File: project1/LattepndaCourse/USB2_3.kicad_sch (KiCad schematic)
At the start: 0 parts

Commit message: Hierachi
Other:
- title: (none) -> practice design
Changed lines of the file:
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@@
 	(generator "eeschema")
 	(generator_version "9.0")
-	(paper "A4")
+	(paper "A2")
+	(title_block
+		(title "practice design")
+		(date "2026-09-30")
+		(rev "1")
+	)
 )

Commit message: USB is done
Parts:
- added C57, C58: 22uF/10V, A_HDJ_Library:C_0603_1608Metric, symbol Device:C_Small
- added C59, C60, C61, C62: 100nF/50V, A_HDJ_Library:C_0603_1608Metric, symbol Device:C_Small
- added D19, D20, D21, D22: ESD9B5.0ST5G, A_HDJ_Library:D_0402_1005Metric, symbol Diode:ESD9B5.0ST5G
- added F1, F2, F3, F4: 6V/1A, A_HDJ_Library:Fuse_0805_2012Metric, symbol Device:Fuse
- added J17: USB_A_Stacked, A_HDJ_Library:USB_A_CUI_UJ2-ADH-TH_Horizontal_Stacked, symbol Connector:USB_A_Stacked
- added J18: USB3_A_Stacked, A_HDJ_Library:USB3_A_Molex_48406-0001_Horizontal_Stacked, symbol Connector:USB3_A_Stacked
- added U13, U14, U15: ULC0524P, A_HDJ_Library:Diodes_UDFN-10_1.0x2.5mm_P0.5mm, symbol Power_Protection:D3V3XA4B10LP
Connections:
- new net: F3.2, J18.1 (VBUS1)
- new net: F4.2, J18.10 (VBUS2)
- new net: F2.2, J17.5 (VBUS2)
- new net: F1.2, J17.1 (VBUS1)
- new net +5V: C57.1, C57.2, C58.1, C58.2, D19.2 (A2), D20.2 (A2), D21.2 (A2), D22.2 (A2), F1.1, F2.1, F3.1, F4.1, J17.4 (GND1), J17.8 (GND2), J17.SH (Shield), J18.13 (GND2), J18.16 (DRAIN2), J18.4 (GND1), J18.7 (DRAIN1), J18.SH (SHIELD), J18.SH (SHIELD), U13.3 (VSS), U13.8 (VSS), U14.3 (VSS), U14.8 (VSS), U15.3 (VSS), U15.8 (VSS)
- new net CON_USB3_SSTX_N: C59.1, J18.8 (SSTX1-), U15.4, U15.7 (NC)
- new net CON_USB3_SSTX_P: C60.1, J18.9 (SSTX1+), U15.5, U15.6 (NC)
- new net CON_USB4_SSTX_N: C61.1, J18.17 (SSTX2-), U15.1, U15.10 (NC)
- new net CON_USB4_SSTX_P: C62.1, J18.18 (SSTX2+), U15.2, U15.9 (NC)
- new net USB3_SSRT_N: J18.5 (SSRX1-), U14.4, U14.7 (NC)
- new net USB3_SSRT_P: J18.6 (SSRX1+), U14.5, U14.6 (NC)
- new net USB3_SSXT_N: C59.2
- new net USB3_SSXT_P: C60.2
- new net USB4_SSRT_N: J18.14 (SSRX2-), U14.1, U14.10 (NC)
- new net USB4_SSRT_P: J18.15 (SSRX2+), U14.2, U14.9 (NC)
- new net USB4_SSXT_N: C61.2
- new net USB4_SSXT_P: C62.2
- new net USB_2_P1+: J18.12 (D2+)
- new net USB_2_P1-: J18.11 (D2-)
- new net USB_2_P2+: J18.3 (D1+)
- new net USB_2_P2-: J18.2 (D1-)
- new net USB_2_P3+: D21.1 (A1), J17.7 (D2+), U13.4, U13.7 (NC)
- new net USB_2_P3-: D22.1 (A1), J17.6 (D2-), U13.5, U13.6 (NC)
- new net USB_2_P5+: D19.1 (A1), J17.3 (D1+), U13.1, U13.10 (NC)
- new net USB_2_P5-: D20.1 (A1), J17.2 (D1-), U13.2, U13.9 (NC)
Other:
- note added: "ESD Protection diods for USB 2.0 data line"
- note added: "USB 2.0"
- note added: "USB 3.0"

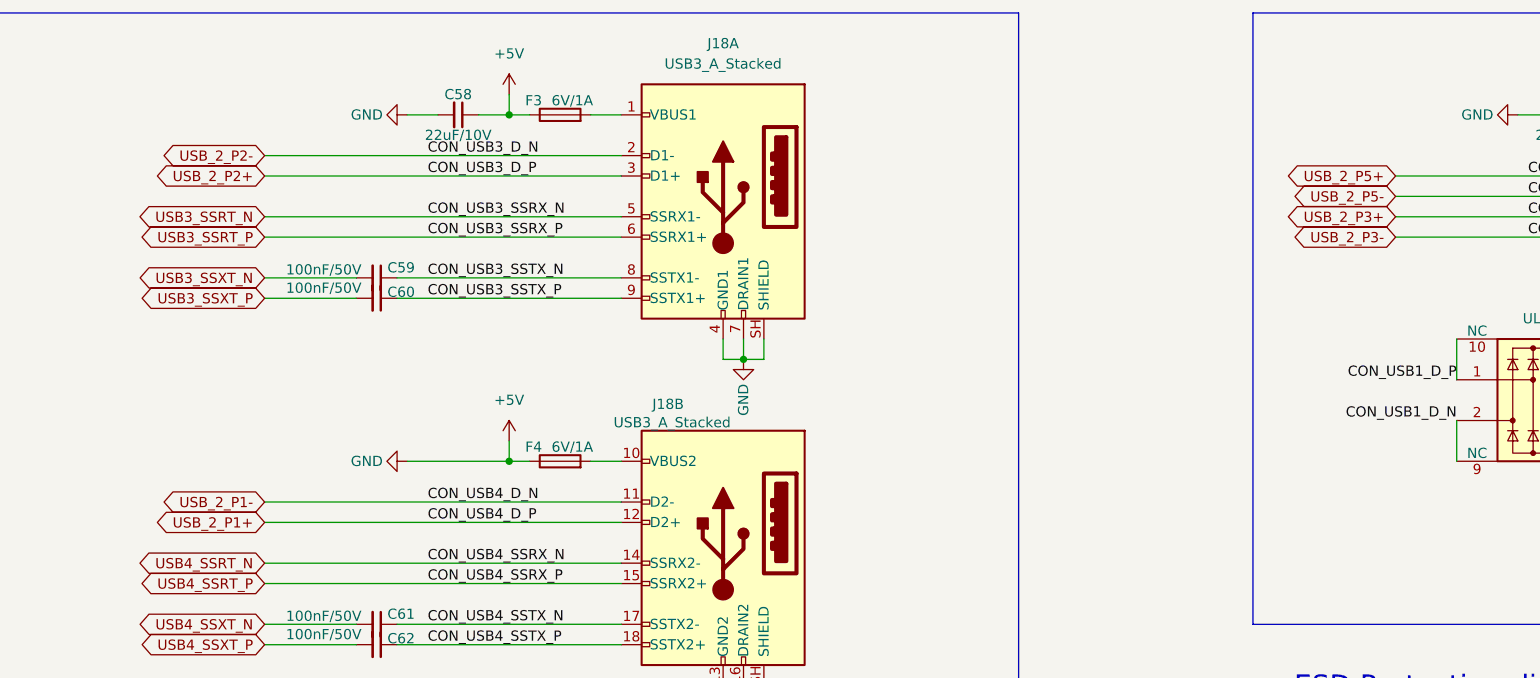
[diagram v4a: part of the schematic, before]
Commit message: Hierachi needs some work
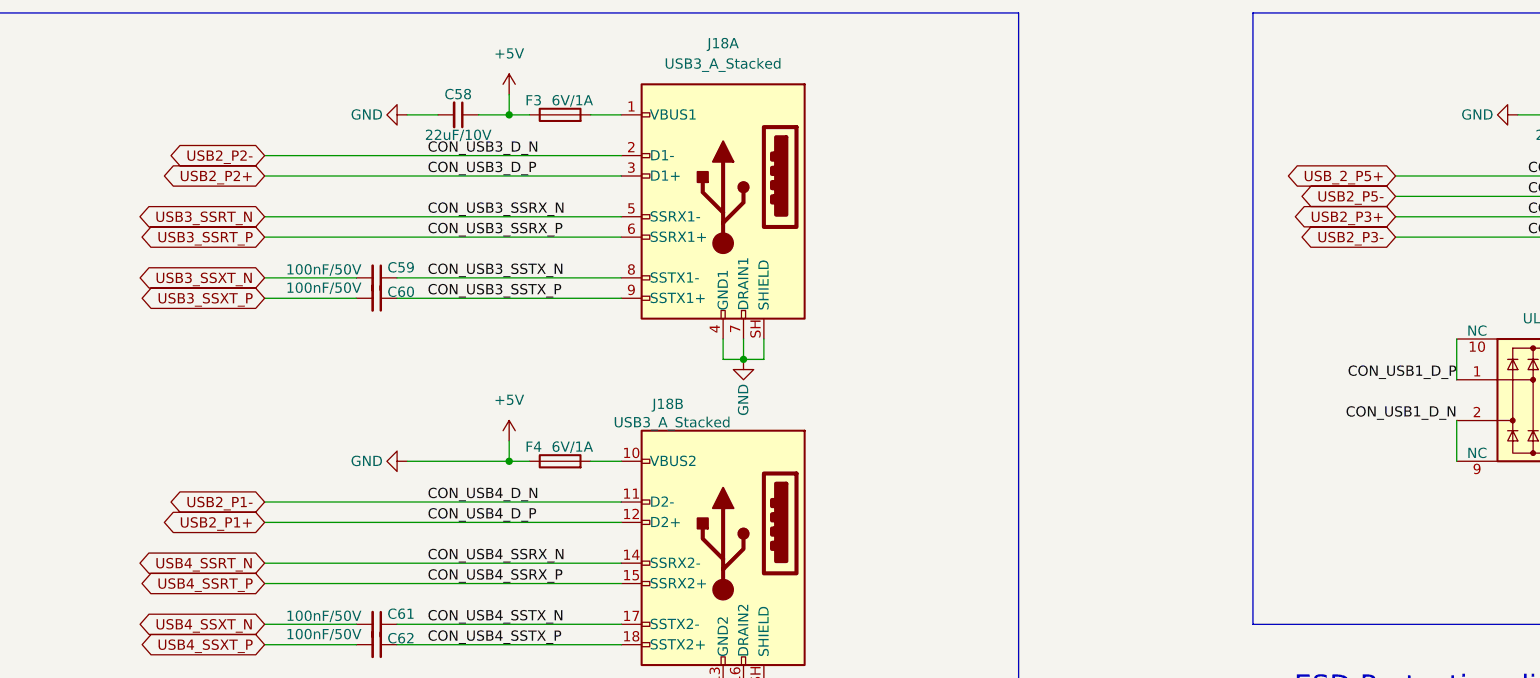
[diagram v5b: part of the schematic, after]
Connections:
- net USB_2_P1+ renamed USB2_P1+
- net USB_2_P1- renamed USB2_P1-
- net USB_2_P2+ renamed USB2_P2+
- net USB_2_P2- renamed USB2_P2-
- net USB_2_P3+ renamed USB2_P3+
- net USB_2_P3- renamed USB2_P3-
- net USB_2_P5- renamed USB2_P5-
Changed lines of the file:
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@@
 		)
 	)
-	(global_label "USB_2_P3+"
+	(global_label "USB2_P3+"
 		(shape bidirectional)
 		(at 196.85 50.8 180)
@@
 		)
 		(property "Intersheetrefs" "${INTERSHEET_REFS}"
-			(at 181.7469 50.8 0)
-			(hide yes)
-			(show_name no)
-			(do_not_autoplace no)
-			(effects
-				(font
-					(size 1.27 1.27)
-				)
-				(justify right)
-			)
-		)
-	)
-	(global_label "USB_2_P1-"
+			(at 182.7145 50.8 0)
+			(hide yes)
+			(show_name no)
+			(do_not_autoplace no)
+			(effects
+				(font
+					(size 1.27 1.27)
+				)
+				(justify right)
+			)
+		)
+	)
+	(global_label "USB2_P1-"
 		(shape bidirectional)
 		(at 55.88 86.36 180)
@@
 		)
 		(property "Intersheetrefs" "${INTERSHEET_REFS}"
-			(at 40.7769 86.36 0)
-			(hide yes)
-			(show_name no)
-			(do_not_autoplace no)
-			(effects
-				(font
-					(size 1.27 1.27)
-				)
-				(justify right)
-			)
-		)
-	)
-	(global_label "USB_2_P5-"
+			(at 41.7445 86.36 0)
+			(hide yes)
+			(show_name no)
+			(do_not_autoplace no)
+			(effects
+				(font
+					(size 1.27 1.27)
+				)
+				(justify right)
+			)
+		)
+	)
+	(global_label "USB2_P5-"
 		(shape bidirectional)
 		(at 196.85 48.26 180)
@@
 		)
 		(property "Intersheetrefs" "${INTERSHEET_REFS}"
-			(at 181.7469 48.26 0)
+			(at 182.7145 48.26 0)
 			(hide yes)
 			(show_name no)
@@
 		)
 	)
-	(global_label "USB_2_P1+"
+	(global_label "USB2_P1+"
 		(shape bidirectional)
 		(at 55.88 88.9 180)
@@
 		)
 		(property "Intersheetrefs" "${INTERSHEET_REFS}"
-			(at 40.7769 88.9 0)
+			(at 41.7445 88.9 0)
 			(hide yes)
 			(show_name no)
@@
 		)
 	)
-	(global_label "USB_2_P2+"
+	(global_label "USB2_P2+"
 		(shape bidirectional)
 		(at 55.88 45.72 180)
@@
 		)
 		(property "Intersheetrefs" "${INTERSHEET_REFS}"
-			(at 40.7769 45.72 0)
+			(at 41.7445 45.72 0)
 			(hide yes)
 			(show_name no)
@@
 		)
 	)
-	(global_label "USB_2_P3-"
+	(global_label "USB2_P3-"
 		(shape bidirectional)
 		(at 196.85 53.34 180)
@@
 		)
 		(property "Intersheetrefs" "${INTERSHEET_REFS}"
-			(at 181.7469 53.34 0)
-			(hide yes)
-			(show_name no)
-			(do_not_autoplace no)
-			(effects
-				(font
-					(size 1.27 1.27)
-				)
-				(justify right)
-			)
-		)
-	)
-	(global_label "USB_2_P2-"
+			(at 182.7145 53.34 0)
+			(hide yes)
+			(show_name no)
+			(do_not_autoplace no)
+			(effects
+				(font
+					(size 1.27 1.27)
+				)
+				(justify right)
+			)
+		)
+	)
+	(global_label "USB2_P2-"
 		(shape bidirectional)
 		(at 55.88 43.18 180)
@@
 		)
 		(property "Intersheetrefs" "${INTERSHEET_REFS}"
-			(at 40.7769 43.18 0)
-			(hide yes)
-			(show_name no)
+			(at 41.7445 43.18 0)
+			(hide yes)
+			(show_name no)
